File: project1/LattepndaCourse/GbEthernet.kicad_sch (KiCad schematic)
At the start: 27 parts, among them J15 RJ45_RB1-125B8G1A, U10 RTL8111H-CG-RH, U11 ULC0524P, U12 ULC0524P, Y1 25MHz

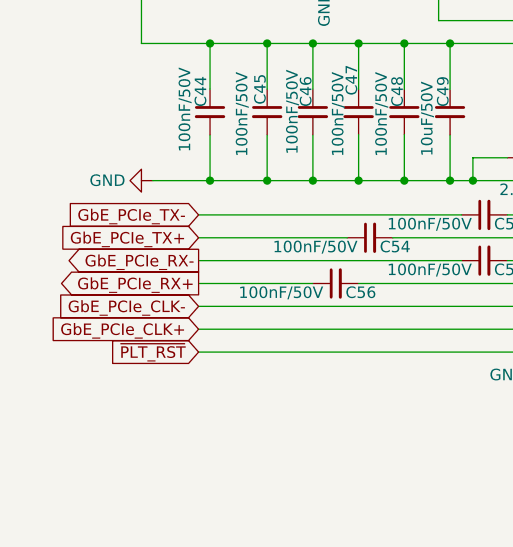
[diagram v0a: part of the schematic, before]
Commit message: fixing Hierachi
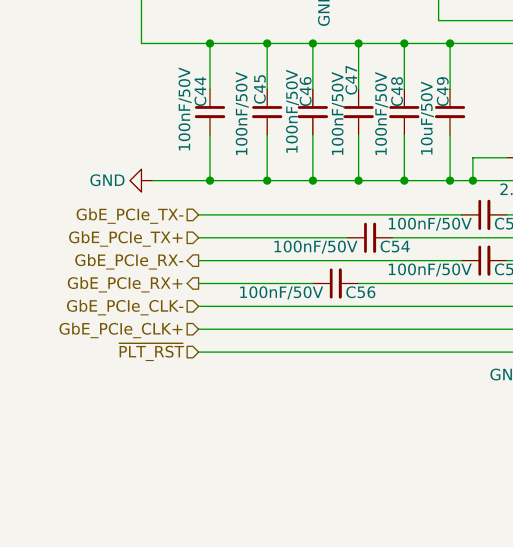
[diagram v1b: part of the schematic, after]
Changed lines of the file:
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@@
 		)
 	)
-	(global_label "GbE_PCIe_CLK+"
-		(shape input)
-		(at 53.34 130.81 180)
-		(fields_autoplaced yes)
+	(hierarchical_label "GbE_PCIe_RX+"
+		(shape output)
+		(at 53.34 125.73 180)
 		(effects
 			(font
@@
 			(justify right)
 		)
-		(property "Intersheetrefs" "${INTERSHEET_REFS}"
-			(at 35.4777 130.81 0)
-			(hide yes)
-			(show_name no)
-			(do_not_autoplace no)
-			(effects
-				(font
-					(size 1.27 1.27)
-				)
-				(justify right)
-			)
-		)
 	)
-	(global_label "~{PLT_RST}"
+	(hierarchical_label "GbE_PCIe_TX+"
 		(shape input)
-		(at 53.34 133.35 180)
-		(fields_autoplaced yes)
+		(at 53.34 120.65 180)
 		(effects
 			(font
@@
 			(justify right)
 		)
-		(property "Intersheetrefs" "${INTERSHEET_REFS}"
-			(at 42.6744 133.35 0)
-			(hide yes)
-			(show_name no)
-			(do_not_autoplace no)
-			(effects
-				(font
-					(size 1.27 1.27)
-				)
-				(justify right)
-			)
-		)
 	)
-	(global_label "GbE_PCIe_RX-"
-		(shape output)
-		(at 53.34 123.19 180)
-		(fields_autoplaced yes)
+	(hierarchical_label "GbE_PCIe_CLK-"
+		(shape input)
+		(at 53.34 128.27 180)
 		(effects
 			(font
@@
 			(justify right)
 		)
-		(property "Intersheetrefs" "${INTERSHEET_REFS}"
-			(at 36.5663 123.19 0)
-			(hide yes)
-			(show_name no)
-			(do_not_autoplace no)
-			(effects
-				(font
-					(size 1.27 1.27)
-				)
-				(justify right)
-			)
-		)
 	)
-	(global_label "GbE_PCIe_CLK-"
+	(hierarchical_label "~{PLT_RST}"
 		(shape input)
-		(at 53.34 128.27 180)
-		(fields_autoplaced yes)
+		(at 53.34 133.35 180)
 		(effects
 			(font
@@
 			(justify right)
 		)
-		(property "Intersheetrefs" "${INTERSHEET_REFS}"
-			(at 35.4777 128.27 0)
-			(hide yes)
-			(show_name no)
-			(do_not_autoplace no)
-			(effects
-				(font
-					(size 1.27 1.27)
-				)
-				(justify right)
-			)
-		)
 	)
-	(global_label "GbE_PCIe_TX+"
+	(hierarchical_label "GbE_PCIe_TX-"
 		(shape input)
-		(at 53.34 120.65 180)
-		(fields_autoplaced yes)
+		(at 53.34 118.11 180)
 		(effects
 			(font
@@
 			(justify right)
 		)
-		(property "Intersheetrefs" "${INTERSHEET_REFS}"
-			(at 36.8687 120.65 0)
-			(hide yes)
-			(show_name no)
-			(do_not_autoplace no)
-			(effects
-				(font
-					(size 1.27 1.27)
-				)
-				(justify right)
-			)
-		)
 	)
-	(global_label "GbE_PCIe_TX-"
-		(shape input)
-		(at 53.34 118.11 180)
-		(fields_autoplaced yes)
+	(hierarchical_label "GbE_PCIe_RX-"
+		(shape output)
+		(at 53.34 123.19 180)
 		(effects
 			(font
@@
 			(justify right)
 		)
-		(property "Intersheetrefs" "${INTERSHEET_REFS}"
-			(at 36.8687 118.11 0)
-			(hide yes)
-			(show_name no)
-			(do_not_autoplace no)
-			(effects
-				(font
-					(size 1.27 1.27)
-				)
-				(justify right)
-			)
-		)
 	)
-	(global_label "GbE_PCIe_RX+"
-		(shape output)
-		(at 53.34 125.73 180)
-		(fields_autoplaced yes)
+	(hierarchical_label "GbE_PCIe_CLK+"
+		(shape input)
+		(at 53.34 130.81 180)
 		(effects
 			(font
@@
 			(justify right)
 		)
-		(property "Intersheetrefs" "${INTERSHEET_REFS}"
-			(at 36.5663 125.73 0)
-			(hide yes)
-			(show_name no)
-			(do_not_autoplace no)
-			(effects
-				(font
-					(size 1.27 1.27)
-				)
-				(justify right)
-			)
-		)
 	)

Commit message: Started routing
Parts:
- Y1: footprint (none) -> A_HDJ_Library:Crystal_SMD_3225-4Pin_3.2x2.5mm
